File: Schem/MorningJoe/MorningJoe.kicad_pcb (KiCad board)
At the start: 4 copper layers, 160 x 64.4 mm, 58 parts, among them J1 DE15_Socket_HighDensity_Mount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, J5 pBITzBus, SW1 SW_Coded_SH-7070, U1 CD74HC139M96, U10 MK4164N, U11 74HC688, U12 MK4164N, U13 MK4164N, U14 MK4164N, U15 MK4164N, U2 TMS9928A, U3 SN74HC273DWR, U4 BAT54JW-7-F, U5 SN74LVC1G19DCKR, U6 THS7314DR, U7 MK4164N, U8 MK4164N, U9 MK4164N, Y1 MP107-E

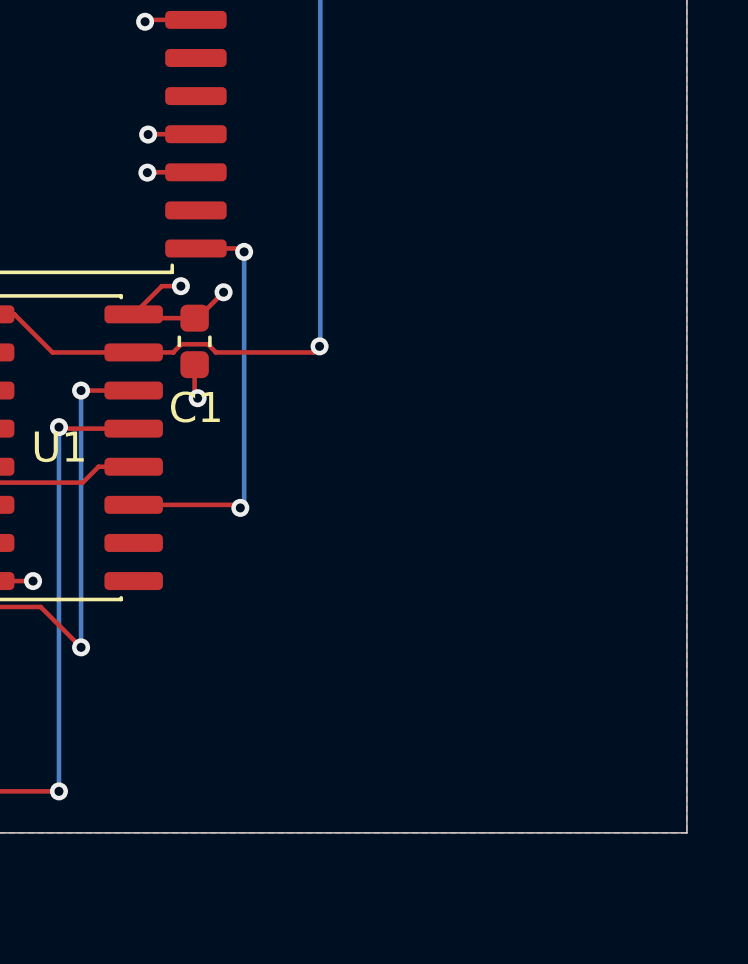
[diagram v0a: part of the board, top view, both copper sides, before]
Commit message: Production Information
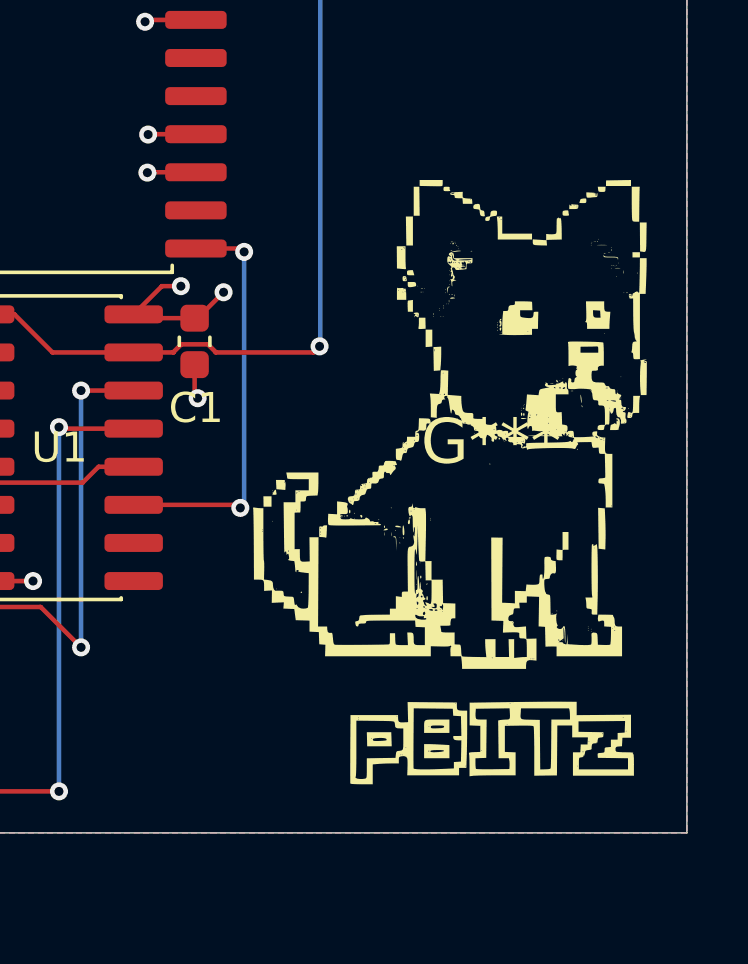
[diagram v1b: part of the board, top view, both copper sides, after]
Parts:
- added G***: LOGO, Footprints:pBITzlogo-Silk, F.Cu at (235.9, 94.5)
